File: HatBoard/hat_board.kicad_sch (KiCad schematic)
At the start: 19 parts, among them J1 DF11 FC Connection, J13 DF11 FC Connection, J2 Conn_01x04, J20 DF11 FC Connection, J21 DF11 FC Connection, U10 VEML7700, U12 DRV2605LDGS, U27 TMP112AIDRLR

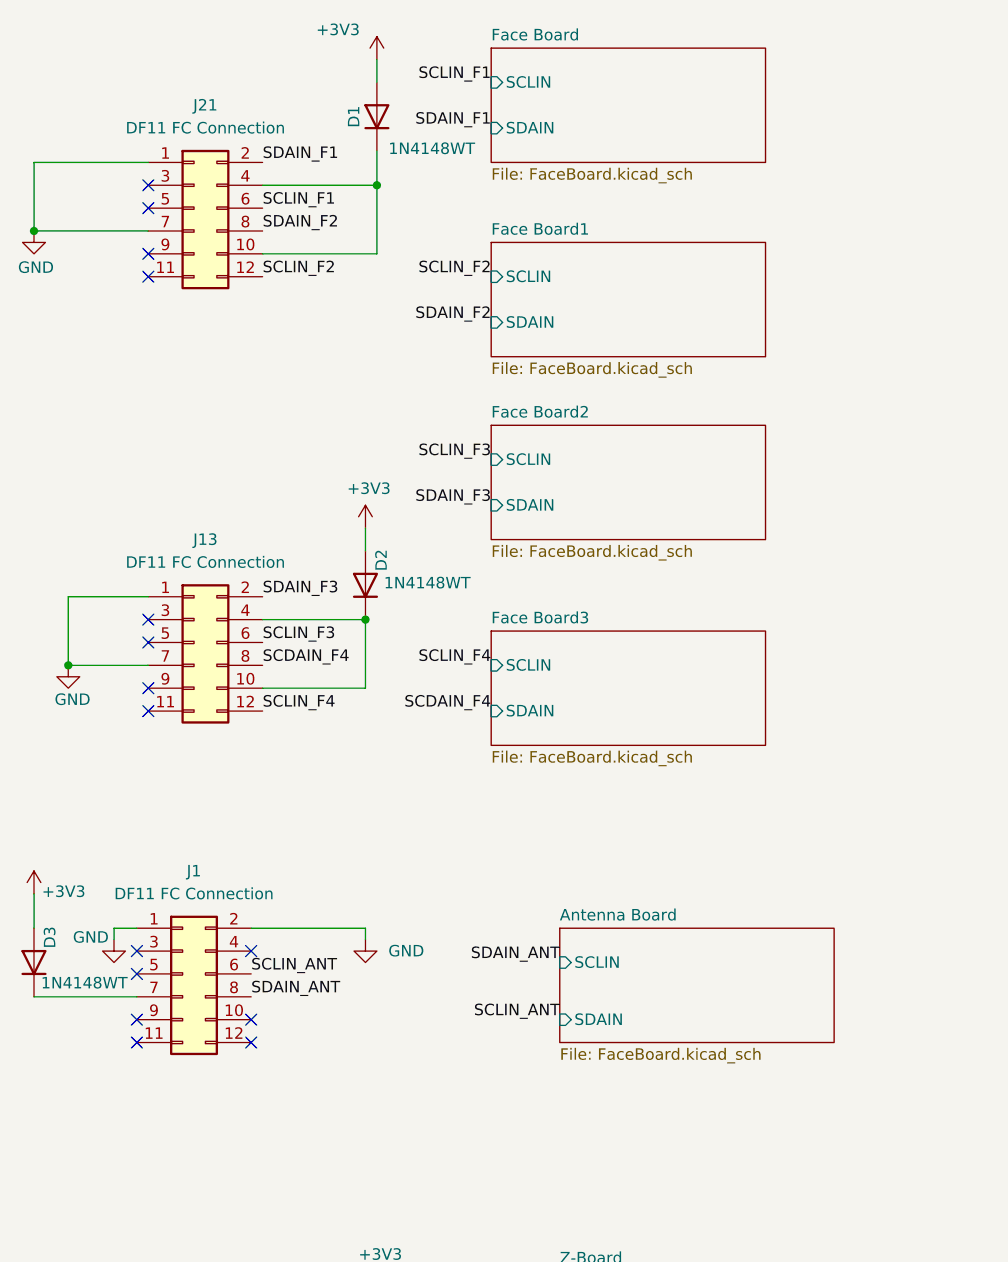
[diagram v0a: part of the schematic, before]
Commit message: from mirror board in schem to bwllo bowrd
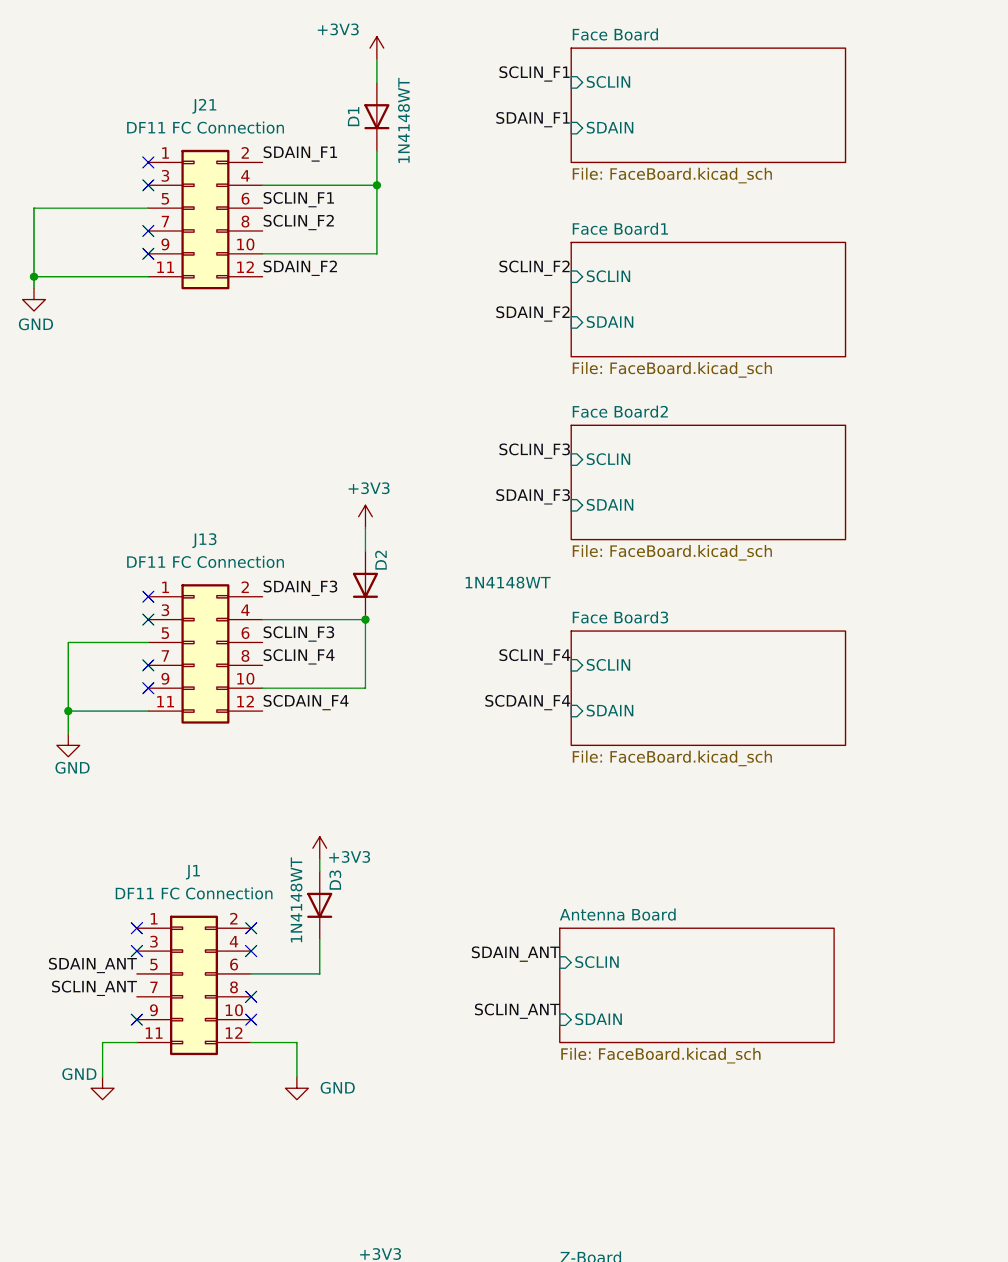
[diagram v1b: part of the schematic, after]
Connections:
- net GND: now also J1.11 (Pin_11), J1.12 (Pin_12), J13.11 (Pin_11), J13.5 (Pin_5), J21.11 (Pin_11), J21.5 (Pin_5); no longer J1.1 (Pin_1), J1.2 (Pin_2), J13.1 (Pin_1), J13.7 (Pin_7), J21.1 (Pin_1), J21.7 (Pin_7)
- net SCDAIN_F4: now also J13.12 (Pin_12); no longer J13.8 (Pin_8)
- net SCLIN_ANT: now also J1.7 (Pin_7); no longer J1.6 (Pin_6)
- net SCLIN_F2: now also J21.8 (Pin_8); no longer J21.12 (Pin_12)
- net SCLIN_F4: now also J13.8 (Pin_8); no longer J13.12 (Pin_12)
- net SDAIN_ANT: now also J1.5 (Pin_5); no longer J1.8 (Pin_8)
- net SDAIN_F2: now also J21.12 (Pin_12); no longer J21.8 (Pin_8)
- net at D3.1 (K): now also J1.6 (Pin_6); no longer J1.7 (Pin_7)
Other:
- moved on the sheet: D3
